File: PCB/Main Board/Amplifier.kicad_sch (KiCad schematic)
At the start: 62 parts

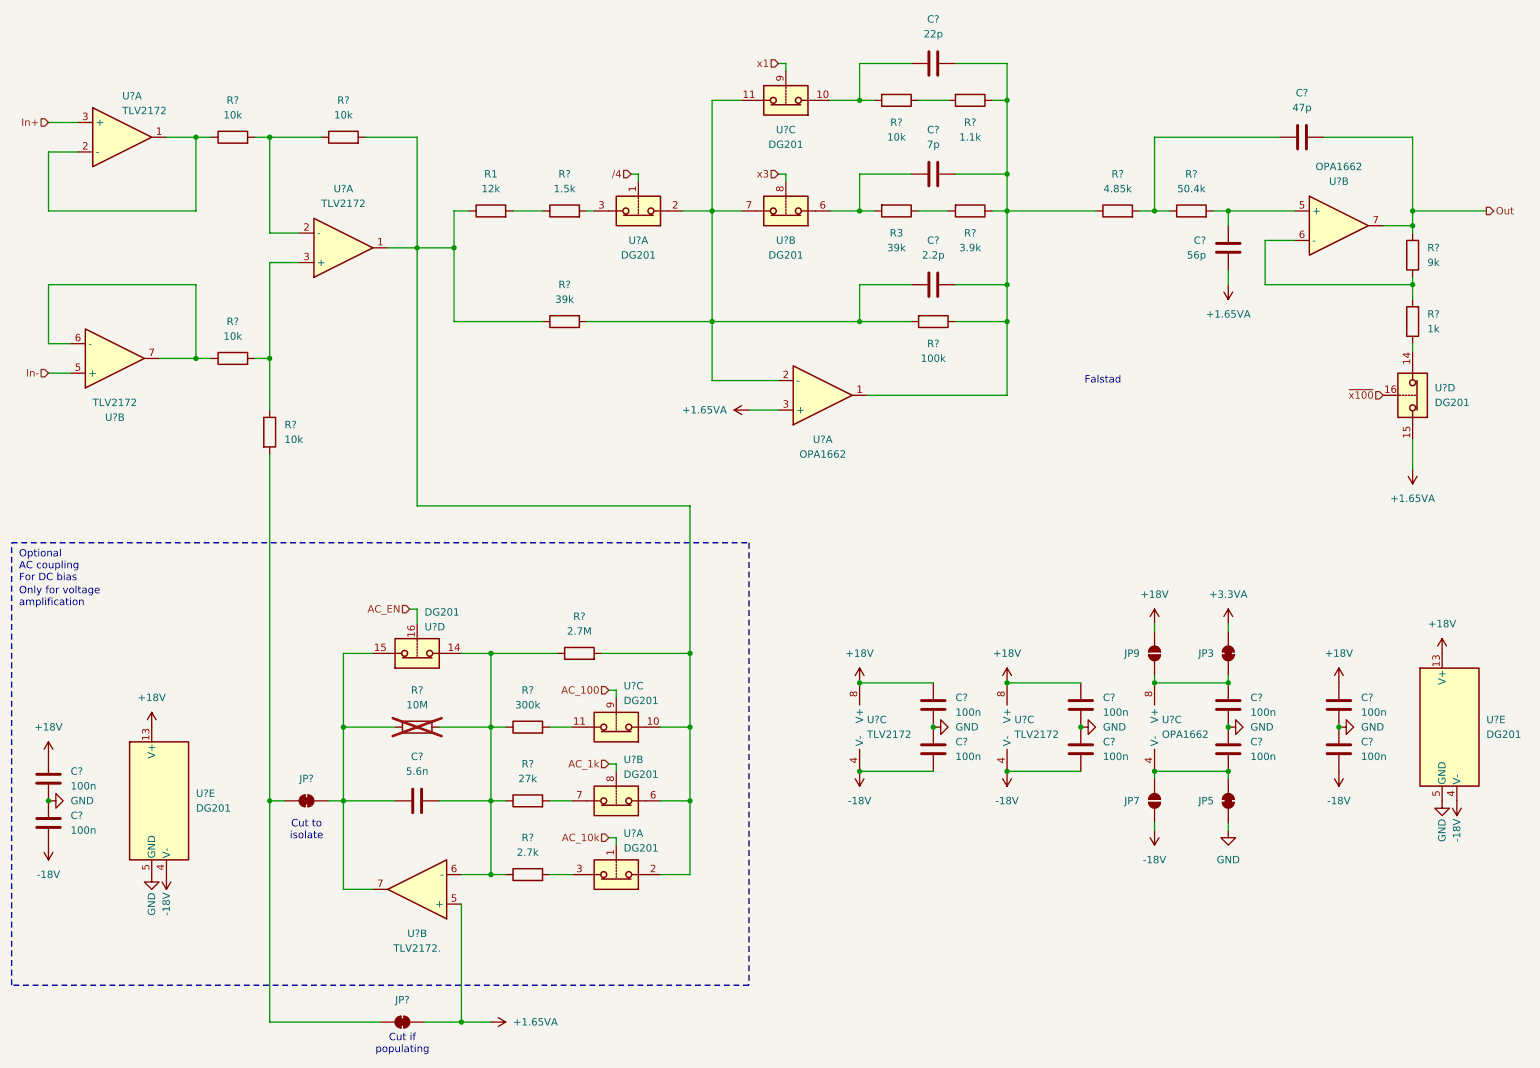
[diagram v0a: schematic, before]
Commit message: Amplifier Switch
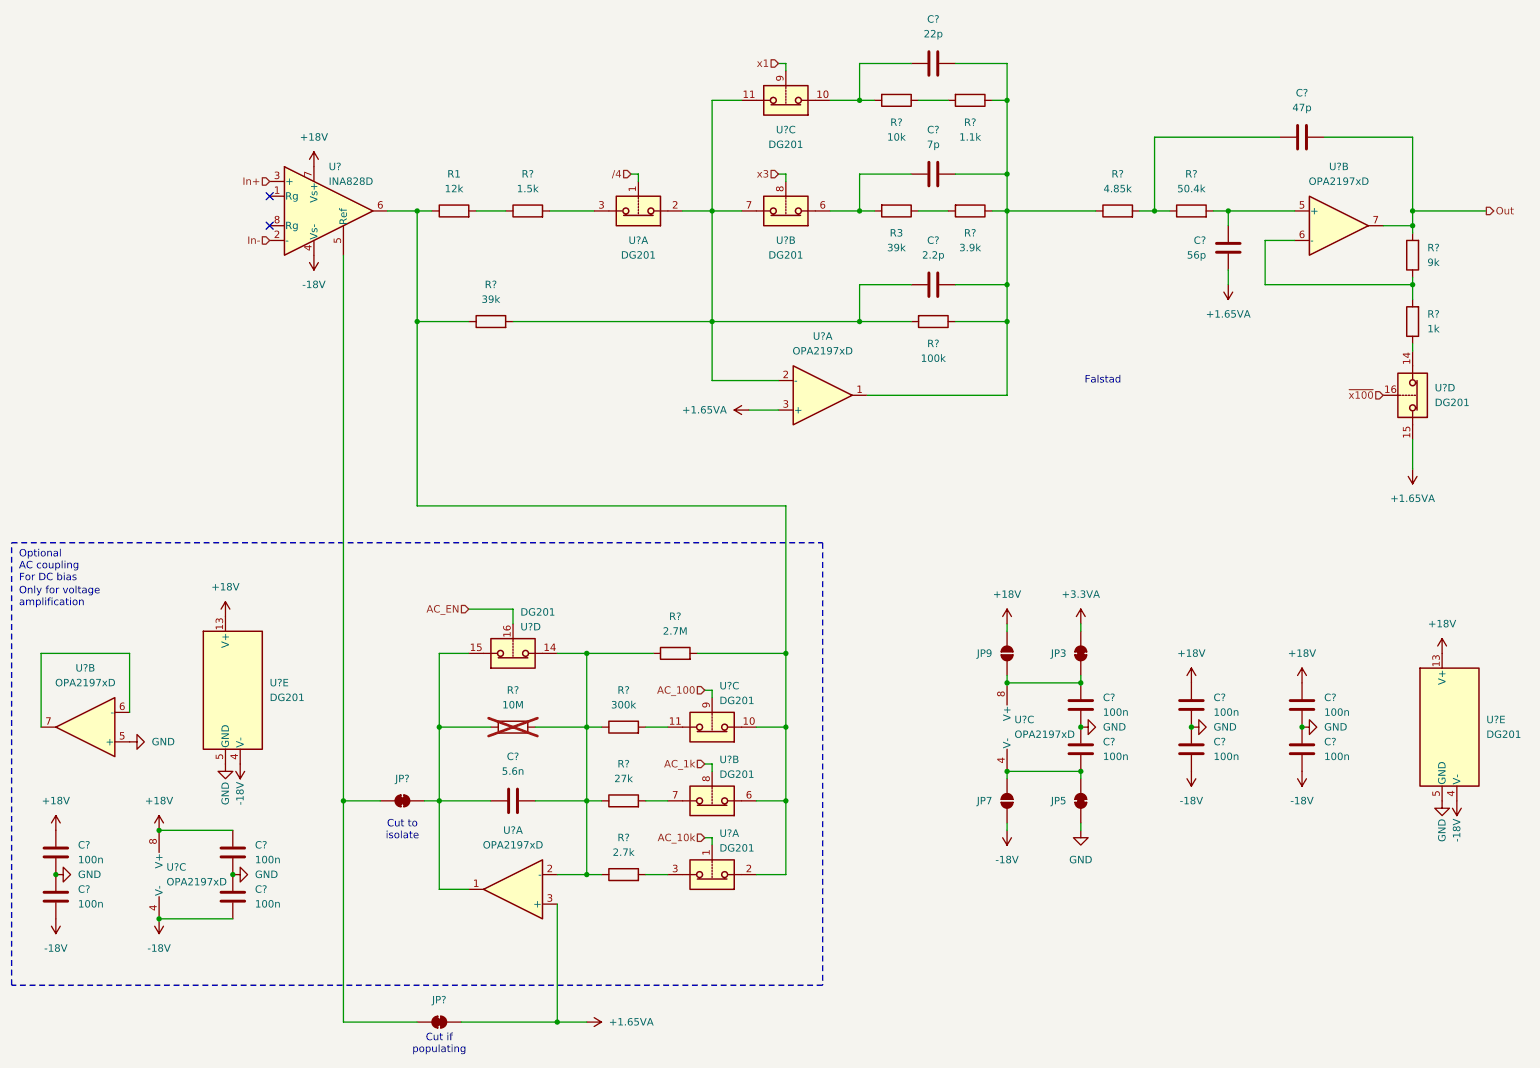
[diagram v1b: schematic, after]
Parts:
- removed R? (x4): 10k, symbol Device:R
- removed U? (x3): OPA1662, Package_SO:SOIC-8_3.9x4.9mm_P1.27mm, symbol Device:Opamp_Dual
- removed U?: TLV2172., Package_SO:SOIC-8_3.9x4.9mm_P1.27mm, symbol Device:Opamp_Dual
- removed U? (x5): TLV2172, Package_SO:SOIC-8_3.9x4.9mm_P1.27mm, symbol Device:Opamp_Dual
- added U? (x6): OPA2197xD, Package_SO:SOIC-8_3.9x4.9mm_P1.27mm, symbol Amplifier_Operational:OPA2197xD
- added U?: INA828D, Package_SO:SOIC-8_3.9x4.9mm_P1.27mm, symbol INA828:INA828D
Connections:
- net +1.65VA: now also U?.3 (+), U?.3 (+)
- net +18V: now also U?.7 (Vs+), U?.8 (V+)
- net -18V: now also U?.4 (V-), U?.4 (Vs-)
- net GND: now also U?.5 (+)
- net In+: now also U?.3 (+)
- net In-: now also U?.2 (-)
- net Out: now also U?.7
- net at C?.2, R?.1, R?.1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: now also U?.2 (-)
- net at C?.1, JP?.2 (B), R?.1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: now also U?.1
- net at C?.1, R?.2, R?.2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: now also U?.2 (-)
- net at C?.2, C?.2, C?.2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: now also U?.1
- net at C?.2, JP5.2 (B), JP7.1 (A): now also U?.4 (V-)
- net at R?.1, R?.2: now also U?.6 (-)
- net at JP?.1 (A), JP?.1 (A): now also U?.5 (Ref)
- net at R1.1, R?.1, R?.2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: now also U?.6
- net at C?.1, R?.2: now also U?.5 (+)
- net at C?.1, JP3.1 (A), JP9.2 (B): now also U?.8 (V+)
- new net: U?.6 (-), U?.7
- no-connect marks 0 -> 2
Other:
- moved on the sheet: C?, JP3, JP5, JP7, JP9, JP?, R1, R?, U?A, U?B, U?C, U?D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
